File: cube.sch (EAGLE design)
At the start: 43 parts, among them CN1 4U#20329, IC3 ATSAMD21E, Q2 reset, U1 AP2112K-3.3

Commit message: made LED7 also a power led
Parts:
- removed BAT: JST-2PH, microbuilder:CON_JST_PH_2PIN
- removed CN1: 4U#20329, microbuilder:USB_MICRO_20329_V2
- removed IC3: ATSAMD21E, microbuilder:ATSAMD21E
- removed JP4: (no value), microbuilder:HEADER-1X576MIL
- removed PWR: green, microbuilder:LED0603_NOOUTLINE
- removed Q2: reset, microbuilder:SWITCH_TACT_SMT4.6X2.8
- removed SWC, SWD: TPB1,27, testpad:TPB1,27
- removed U$11, U$12: MOUNTINGHOLE2.0, microbuilder:MOUNTINGHOLE2.0
- removed U$8: FIDUCIAL_1MM, microbuilder:FIDUCIAL_1MM
- added C10, C15: 10uF, microbuilder:CAP_CERAMIC0805-NOOUTLINE
- added C11, C12, C13, C14, C16, C7: 1uF, microbuilder:CAP_CERAMIC0603_NO
- added C4, C6: 10µF, microbuilder:CAP_CERAMIC0805-NOOUTLINE
- added C5, C9: 22pF, microbuilder:CAP_CERAMIC0603_NO
- added CHG: ORANGE, microbuilder:LED0805_NOOUTLINE
- added D+, D-: TPB1,27, testpad:TPB1,27
- added JP2: (no value), pinhead:PINHD-2X2
- added L2: 10uH, microbuilder:INDUCTOR
- added PWR_LED7: green, microbuilder:LED0603_NOOUTLINE
- added Q1, Q3: DMG341, microbuilder:MOSFET-P
- added R10, R11, R5, R6: 10K, microbuilder:RESISTOR_0603_NOOUT
- added R7: 2.2K, microbuilder:RESISTOR_0603_NOOUT
- added R8: 10K\, microbuilder:RESISTOR_0603_NOOUT
- added R9: 100K, microbuilder:RESISTOR_4PACK_NO
- added SJ1: (no value), microbuilder:SOLDERJUMPERCLOSED
- added SW1: KMR2, microbuilder:SWITCH_TACT_SMT4.6X2.8
- added TP1, TP2: (no value), microbuilder:TESTPOINTROUND1.5MM
- added U$24: ATSAMD51J, microbuilder:ATSAMD51J
- added U$31, U$32: MOUNTINGHOLE2.5, microbuilder:MOUNTINGHOLE2.5
- added U$34, U$35: FIDUCIAL_1MM, microbuilder:FIDUCIAL_1MM
- added U2: AP2112-3.3, microbuilder:VREG_SOT23-5
- added U3: MCP73831T-2ACI/OT, microbuilder:MCP73831/2
- added U4: 2MB Flash, microbuilder:SPIFLASH_8PINUX
- added X1: JSTPH, microbuilder:CON_JST_PH_2PIN
- added X2: 32.768, adafruit2:XTAL-3.2X1.5
- added X3: microUSB, microbuilder:USB_MICRO_20329_V2
- C3: value 1uF -> 10µF; device microbuilder:CAP_CERAMIC0603_NO -> microbuilder:CAP_CERAMIC0805-NOOUTLINE
- D8: value (none) -> MBR120; device microbuilder:LED0603_NOOUTLINE -> microbuilder:DIODE-SCHOTTKYSOD-123
- JP1: device microbuilder:HEADER-2X3 -> microbuilder:HEADER-1X16ROUND
- JP3: device microbuilder:HEADER-1X576MIL -> microbuilder:HEADER-1X12
- L: value red -> RED; device microbuilder:LED0603_NOOUTLINE -> microbuilder:LED0805_NOOUTLINE
- LED1: value AP102-2020 -> WS2812B3535; device microbuilder:APA1022020 -> microbuilder:WS2812B3535
- R3: value 1.5K -> 1K
- R4: value 10K -> 500
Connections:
- net VOUT renamed VIN
- removed net D0_A4_PA08_SDA: IC3.PA08/I2C/AIN16/SERCOM0+2.0/I2SD1, JP4.4
- removed net D1_A0_PA02: IC3.PA02/EINT2/AIN0/Y0/VOUT, JP4.3
- removed net D2_A1_PA09_SCL_MISO: IC3.PA09/I2C/I9/AIN17/SERCOM0+2.1/I2SMC, JP4.2
- removed net D3_A3_PA07_RXD_SCK: IC3.PA07/I7/AIN7/SERCOM0.3/I2SD0, JP3.4
- removed net D4_A2_PA06_TXD_MOSI: IC3.PA06/EINT6/AIN6/SERCOM0.2, JP3.3
- removed net LED7: R2G$4.1, U$7.PA04/I4/VREFB/AIN2/Y2/SERCOM0.2+0.0
- removed net LED_A7: D8.A, R2G$4.2
- removed net N$6: PWR.A, R4.1
- removed net PA22/I2C/I6/X6/Y12/SERCOM1.0+2.0: U$7.PA22/I2C/I6/X6/Y12/SERCOM1.0+2.0
- removed net SAO_GPIO1: JP1.1
- removed net SAO_GPIO2: JP1.2
- removed net VDDCORE: C3.1, IC3.VDDCORE
- new net +3V3: C10.1, C11.1, C12.1, C3.1, C7.1, JP1.15, LED1.VDD, R11.1, R5.2, R6.1, SJ1.2, U$24G$1.PA07/I7/AIN7/SERCOM0.3, U$24G$3.VDDANA, U$24G$3.VDDIO_0, U$24G$3.VDDIO_1, U$24G$3.VDDIO_2, U$24G$3.VDDIO_3, U2.OUT, U4.VCC
- new net A0: JP1.12, U$24G$1.PA02/EINT2/AIN0/VOUT0
- new net A1: JP1.11, U$24G$1.PA05/I5/AIN5/VOUT1/SERCOM0.1
- new net A2: JP1.10, U$24G$2.PB08/I8/AIN2/SERCOM4.0
- new net A4: JP1.8, U$24G$1.PA04/I4/VREFB/AIN4/SERCOM0.0
- new net A5: JP1.7, U$24G$1.PA06/I6/VREFC/AIN6/SERCOM0.2
- new net AREF: C14.1, JP1.14, SJ1.1, U$24G$1.PA03/I3/VREFA/AIN1
- new net D10: JP3.7, U$24G$1.PA20/I4/SERCOM3+5.2/I2SFS0
- new net D11: JP3.6, U$24G$1.PA21/I5/SERCOM3+5.3/I2SDO
- new net D12: JP3.5, U$24G$1.PA22/I2C/16/SERCOM3.0+5.1/I2SDI
- new net D13: JP3.4, R7.1, U$24G$1.PA23/I2C/I7/SERCOM3.1+5.0/SOF/I2SFS1
- new net D4: JP1.1, U$24G$1.PA14/I14/SERCOM2+4.2
- new net D5: JP3.10, U$24G$1.PA16/I2C/I0/SERCOM1.0+3.1
- new net D6: JP3.9, U$24G$1.PA18/I2/SERCOM1+3.2
- new net D8_NEOPIX: LED1.DI, U$24G$2.PB03/I3/AIN15/SERCOM5.1
- new net D9: JP3.8, U$24G$1.PA19/I3/SERCOM1+3.3
- new net EN: JP3.2, R10.1, U2.EN
- new net LED7_PWR: Q1.G, U$7.PA04/I4/VREFB/AIN2/Y2/SERCOM0.2+0.0
- new net MISO: JP1.4, U$24G$2.PB22/I6/SERCOM1+5.2
- new net MOSI: JP1.5, U$24G$2.PB23/I7/SERCOM1+5.3
- new net N$11: L2.2, U$24G$3.VSW
- new net N$36: Q1.D, R4.1
- new net N$9: C9.1, U$24G$1.PA01/EINT1/SERCOM1.1, X2.P$2
- new net QSPI_CS: R5.1, U$24G$2.PB11/I11/SERCOM4.3/I2SFS1, U4.SSEL
- new net QSPI_DATA[0]: U$24G$1.PA08/I2C/AIN8/SERCOM0.0+2.1/I2SMCK, U4.MOSI
- new net QSPI_DATA[1]: U$24G$1.PA09/I2C/I9/AIN9/SERCOM0.1+2.0/I2SFS0, U4.MISO
- new net QSPI_DATA[2]: U$24G$1.PA10/I10/AIN10/SERCOM0+2.2/I2SCK, U4.WP#/IO2
- new net QSPI_DATA[3]: U$24G$1.PA11/I11/AIN11/SERCOM0+2.3/I2SDO, U4.HOLD#/IO3
- new net QSPI_SCK: U$24G$2.PB10/I10/SERCOM4.2/I2SDI, U4.SCK
- new net RX_D0: JP1.3, U$24G$2.PB17/SERCOM5.1/I2SMCK0
- new net SCK: JP1.6, U$24G$1.PA17/I2C/I1/SERCOM1.1+3.0
- new net SCL: JP3.11, U$24G$1.PA13/I13/I2C/SERCOM2.1+4.0
- new net SDA: JP3.12, U$24G$1.PA12/I12/I2C/SERCOM2.0+4.1
- new net SWCLK: R11.2, TP1.P$1, U$24G$1.PA30/I14/SERCOM1.2/SWCLK
- new net SWDIO: TP2.P$1, U$24G$1.PA31/I15/SERCOM1.3/SWDIO
- new net TX_D1: JP1.2, U$24G$2.PB16/I0/SERCOM5.0/I2SCK0
- new net VDDCORE1: C15.1, C16.1, L2.1, U$24G$3.VDDCORE
- new net VHI: C6.1, D8.C, Q3.S, R10.2, U2.IN
- new net VHI1: PWR_LED7.A, Q1.S
- new net V_DIV: R9G$1.1, R9G$2.1, U$24G$2.PB01/I1/AIN13/SERCOM5.3
- net !RESET: now also C13.2, JP1.16, R6.2, SW1.P, SW1.P1, U$24G$3.!RESET; no longer IC3./RESET, JP3.5, Q2.P, Q2.P1
- net 3.3V: no longer IC3.VDDA, IC3.VDDIN, JP4.1, LED1.VDD
- net A3: now also JP1.9, U$24G$2.PB09/I9/AIN3/SERCOM4.1; no longer IC3.PA00/EINT0/SERCOM1.0, LED1.DI
- net D+: now also D+.TP, U$24G$1.PA25/19/SERCOM3+5.3/D+, X3.D+; no longer CN1.D+, IC3.PA25/I13/SERCOM3+5.3/D+
- net D-: now also D-.TP, U$24G$1.PA24/I8/SERCOM3+5.2/D-, X3.D-; no longer CN1.D-, IC3.PA24/I12/SERCOM3+5.2/D-
- net GND: now also C10.2, C11.2, C12.2, C13.1, C14.2, C15.2, C16.2, C4.2, C5.2, C6.2, C7.2, C9.2, JP1.13, JP2.1, PWR_LED7.C, R8.2, R9G$2.2, R9G$3.1, SW1.S, SW1.S1, U$24G$3.GND_0, U$24G$3.GND_1, U$24G$3.GND_2, U$24G$3.GND_3, U$24G$3.GND_4, U2.GND, U3.VSS, U4.VSS, X1.1, X3.GND; no longer BAT.1, CN1.GND, D8.C, IC3.GND, IC3.GNDA, JP1.6, JP3.2, PWR.C, Q2.S, Q2.S1
- net N$1: now also CHG.C; no longer L.A
- net N$2: now also L.A, R7.2; no longer IC3.PA10/I10/AIN18/SERCOM0+2.2/I2SCK, R3.2
- net N$3: now also R3.2, U3.STAT; no longer IC3.PA30/I10/SECOM1.2/SWCLK, SWC.TP
- net N$4: now also R8.1, U3.PROG; no longer IC3.PA31/I11/SECOM1.3/SWDIO, SWD.TP
- net N$8: now also C5.1, U$24G$1.PA00/EINT0/SERCOM1.0, X2.P$1; no longer IC3.PA01/EINT1/SERCOM1.1, LED1.CKI
- net SAO_SCL: now also JP2.3; no longer JP1.4
- net SAO_SDA: now also JP2.4; no longer JP1.3
- net SAO_VDD: now also JP2.2; no longer JP1.5
- net VBAT: now also C4.1, Q3.D, R9G$1.2, U3.VBAT, X1.2; no longer BAT.2
- net VBUS: now also CHG.A, D8.A, JP3.3, Q3.G, R9G$3.2, U3.VDD, X3.VBUS; no longer CN1.VBUS, JP4.5
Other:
- note added: "1.0K = 1000mA"
- note added: "10K = 100mA"
- note added: "2.0K = 500mA"
- note added: "5.0K = 200mA"
- note added: "BREAKOUTS"
- note added: "CAN0_RX"
- note added: "CAN0_TX"
- note added: "CAN1_RX"
- note added: "CAN1_TX"
- note added: "DAC0"
- note added: "DAC1"
- note added: "PCC: DEN1: SDA DEN2: SCL CLK: D6 D0: D11 D1: D13 D2: D10 D3: D12 D4: MISO D5: D5 D6: MOSI D7: SCK SPI: SERCOM1 DOPO = 0x3, SCK.1 & MO.3, MI.2 I2C: SERCOM2 or 4 UART: SERCOM5, TX on .0 & RX on .1 SPI Flash: QSPI (dual io) I2S: SCK0: A2 FS0: MISO SDI: MOSI SDO: D5 TCC1: WO0: D11 WO1: D13 WO2: D10 WO3: D12 WO4: MISO WO5: D5 WO6: MOSI WO7: SCK"
- note added: "PCCD0"
- note added: "PCCD1"
- note added: "PCCD2"
- note added: "PCCD3"
- note added: "PCCD4"
- note added: "PCCD5"
- note added: "PCCD6"
- note added: "PCCD7"
- note added: "PCCDEN1"
- note added: "PCCDEN2"
- note added: "PCCLK"
- note added: "POWER AND FILTERING"
- note added: "RED LED"
- note added: "RESET"
- note added: "USB AND BATTERY CHARGING"
- note added: "p-channel"
- note removed: "Adafruit Trinket M0"
- note removed: "CC 2.5 BY-SA"
- note removed: "http://adafruit.com/products/3500"

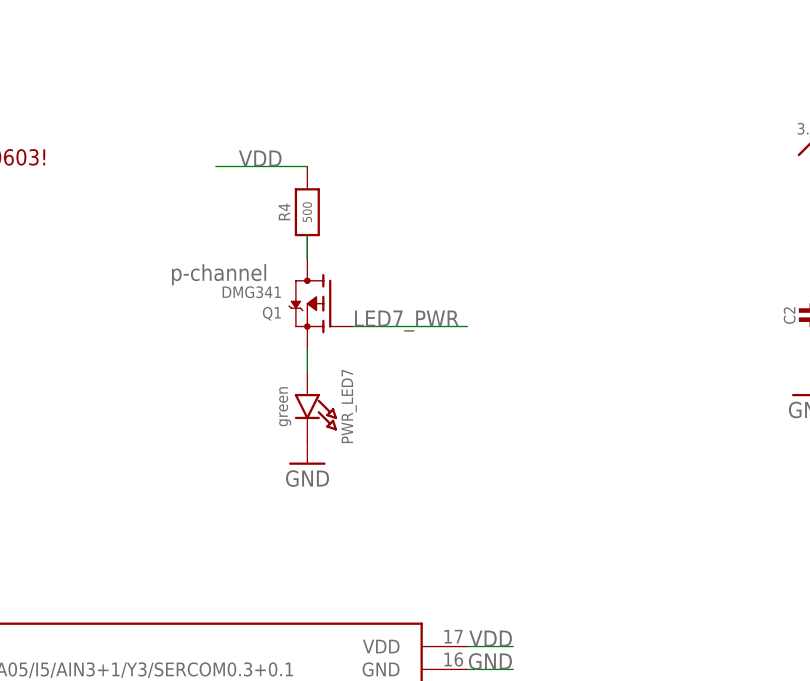
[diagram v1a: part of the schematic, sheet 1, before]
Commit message: updtes with suggestion from cgrover
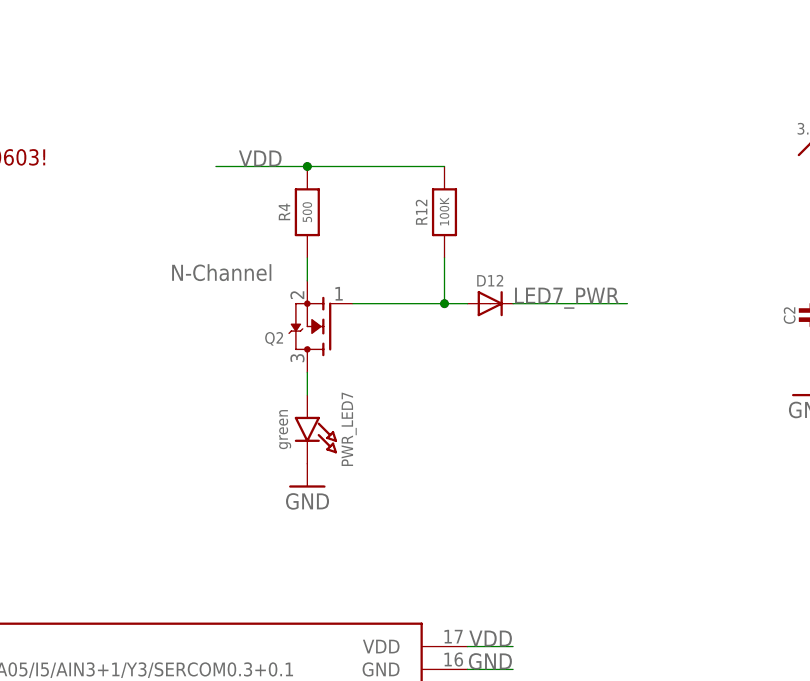
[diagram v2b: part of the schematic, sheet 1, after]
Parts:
- removed Q1: DMG341, microbuilder:MOSFET-P
- added D12: (no value), microbuilder:DIODESOD-323
- added Q2: (no value), microbuilder:MOSFET-NREFLOW
- added R12: 100K, microbuilder:RESISTOR_0603_NOOUT
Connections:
- new net N$6: D12.A, Q2.G, R12.1
- net LED7_PWR: now also D12.C; no longer Q1.G
- net N$36: now also Q2.S; no longer Q1.D
- net VDD: now also R12.2
- net VHI1: now also Q2.D; no longer Q1.S
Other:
- note added: "N-Channel"
- note removed: "p-channel"
- moved on the sheet: PWR_LED7
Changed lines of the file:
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@@
 <part name="+3V3" library="supply1" library_urn="urn:adsk.eagle:library:371" deviceset="+3V3" device=""/>
 <part name="U$41" library="microbuilder" deviceset="FRAME_A3_ADAFRUIT" device=""/>
-<part name="Q1" library="microbuilder" deviceset="MOSFET-P" device="" value="DMG341"/>
+<part name="Q2" library="microbuilder" deviceset="MOSFET-N" device="REFLOW"/>
+<part name="R12" library="microbuilder" deviceset="RESISTOR" device="_0603_NOOUT" value="100K"/>
+<part name="D12" library="microbuilder" deviceset="DIODE" device="SOD-323"/>
 </parts>
 <sheets>
@@
 0x2  PAD[3] PAD[1] PAD[2]   System configuration
 0x3  PAD[0] PAD[3] PAD[1]   System configuration</text>
-<text x="10.16" y="248.92" size="1.778" layer="95">p-channel</text>
+<text x="10.16" y="248.92" size="1.778" layer="95">N-Channel</text>
 </plain>
 <instances>
@@
 <attribute name="VALUE" x="25.4" y="256.54" size="1.016" layer="96" font="vector" ratio="15" rot="R90" align="center"/>
 </instance>
-<instance part="PWR_LED7" gate="G$1" x="25.4" y="233.68" smashed="yes" rot="R270">
-<attribute name="NAME" x="29.845" y="234.95" size="1.27" layer="95" rot="R270" align="center"/>
-<attribute name="VALUE" x="22.606" y="234.95" size="1.27" layer="96" rot="R270" align="center"/>
-</instance>
-<instance part="GND6" gate="1" x="25.4" y="228.6" smashed="yes" rot="MR0">
-<attribute name="VALUE" x="27.94" y="226.06" size="1.778" layer="96" rot="MR0"/>
+<instance part="PWR_LED7" gate="G$1" x="25.4" y="231.14" smashed="yes" rot="R270">
+<attribute name="NAME" x="29.845" y="232.41" size="1.27" layer="95" rot="R270" align="center"/>
+<attribute name="VALUE" x="22.606" y="232.41" size="1.27" layer="96" rot="R270" align="center"/>
+</instance>
+<instance part="GND6" gate="1" x="25.4" y="226.06" smashed="yes" rot="MR0">
+<attribute name="VALUE" x="27.94" y="223.52" size="1.778" layer="96" rot="MR0"/>
 </instance>
 <instance part="D9" gate="G$1" x="-71.12" y="254" smashed="yes" rot="R270">
@@
 <attribute name="VALUE" x="-120.65" y="203.2" size="1.778" layer="96"/>
 </instance>
-<instance part="Q1" gate="G$1" x="25.4" y="246.38" smashed="yes" rot="R180">
-<attribute name="VALUE" x="22.606" y="248.285" size="1.27" layer="96" rot="R180"/>
-<attribute name="NAME" x="22.606" y="245.999" size="1.27" layer="95" rot="R180"/>
+<instance part="Q2" gate="G$1" x="27.94" y="243.84" smashed="yes" rot="R180">
+<attribute name="NAME" x="22.86" y="243.205" size="1.27" layer="95" rot="R180"/>
+<attribute name="VALUE" x="22.86" y="245.11" size="1.27" layer="96" rot="R180"/>
+</instance>
+<instance part="R12" gate="G$1" x="40.64" y="256.54" smashed="yes" rot="R90">
+<attribute name="NAME" x="38.1" y="256.54" size="1.27" layer="95" font="vector" rot="R90" align="center"/>
+<attribute name="VALUE" x="40.64" y="256.54" size="1.016" layer="96" font="vector" ratio="15" rot="R90" align="center"/>
+</instance>
+<instance part="D12" gate="G$1" x="45.72" y="246.38" smashed="yes">
+<attribute name="NAME" x="45.72" y="248.92" size="1.27" layer="95" align="center"/>
+<attribute name="VALUE" x="45.72" y="243.88" size="1.27" layer="96" align="center"/>
 </instance>
 </instances>
@@
 <wire x1="25.4" y1="261.62" x2="15.24" y2="261.62" width="0.1524" layer="91"/>
 <label x="17.78" y="261.62" size="1.778" layer="95"/>
+<pinref part="R12" gate="G$1" pin="2"/>
+<wire x1="40.64" y1="261.62" x2="25.4" y2="261.62" width="0.1524" layer="91"/>
+<junction x="25.4" y="261.62"/>
 </segment>
 </net>
@@
 <net name="VHI1" class="0">
 <segment>
-<pinref part="Q1" gate="G$1" pin="S"/>
-<wire x1="25.4" y1="241.3" x2="25.4" y2="238.76" width="0.1524" layer="91"/>
 <pinref part="PWR_LED7" gate="G$1" pin="A"/>
+<pinref part="Q2" gate="G$1" pin="D"/>
+<wire x1="25.4" y1="236.22" x2="25.4" y2="238.76" width="0.1524" layer="91"/>
 </segment>
 </net>
@@
 </segment>
 <segment>
-<pinref part="Q1" gate="G$1" pin="G"/>
-<wire x1="30.48" y1="243.84" x2="43.18" y2="243.84" width="0.1524" layer="91"/>
-<label x="30.48" y="243.84" size="1.778" layer="95"/>
+<wire x1="48.26" y1="246.38" x2="60.96" y2="246.38" width="0.1524" layer="91"/>
+<label x="48.26" y="246.38" size="1.778" layer="95"/>
+<pinref part="D12" gate="G$1" pin="C"/>
 </segment>
 </net>
 <net name="N$36" class="1">
 <segment>
-<pinref part="Q1" gate="G$1" pin="D"/>
 <pinref part="R4" gate="G$1" pin="1"/>
-<wire x1="25.4" y1="254" x2="25.4" y2="251.46" width="0.1524" layer="91"/>
-</segment>
-</net>
+<pinref part="Q2" gate="G$1" pin="S"/>
+<wire x1="25.4" y1="248.92" x2="25.4" y2="251.46" width="0.1524" layer="91"/>
+</segment>
+</net>
+<net name="N$6" class="0">
+<segment>
+<pinref part="Q2" gate="G$1" pin="G"/>
+<wire x1="30.48" y1="246.38" x2="40.64" y2="246.38" width="0.1524" layer="91"/>
+<pinref part="R12" gate="G$1" pin="1"/>
+<wire x1="40.64" y1="246.38" x2="43.18" y2="246.38" width="0.1524" layer="91"/>
+<wire x1="40.64" y1="251.46" x2="40.64" y2="246.38" width="0.1524" layer="91"/>
+<junction x="40.64" y="246.38"/>
+<pinref part="D12" gate="G$1" pin="A"/>
+</segment>
+</net>
